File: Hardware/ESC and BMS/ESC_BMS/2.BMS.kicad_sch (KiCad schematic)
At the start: 46 parts, among them Q10 NTD25P03LT4G, Q8 NTD25P03LT4G, Q9 NMOS, SW2 SW_SPST, U12 BQ2969T, U13 74AUC2G08, U14 TPS25926, U16 BQ2057

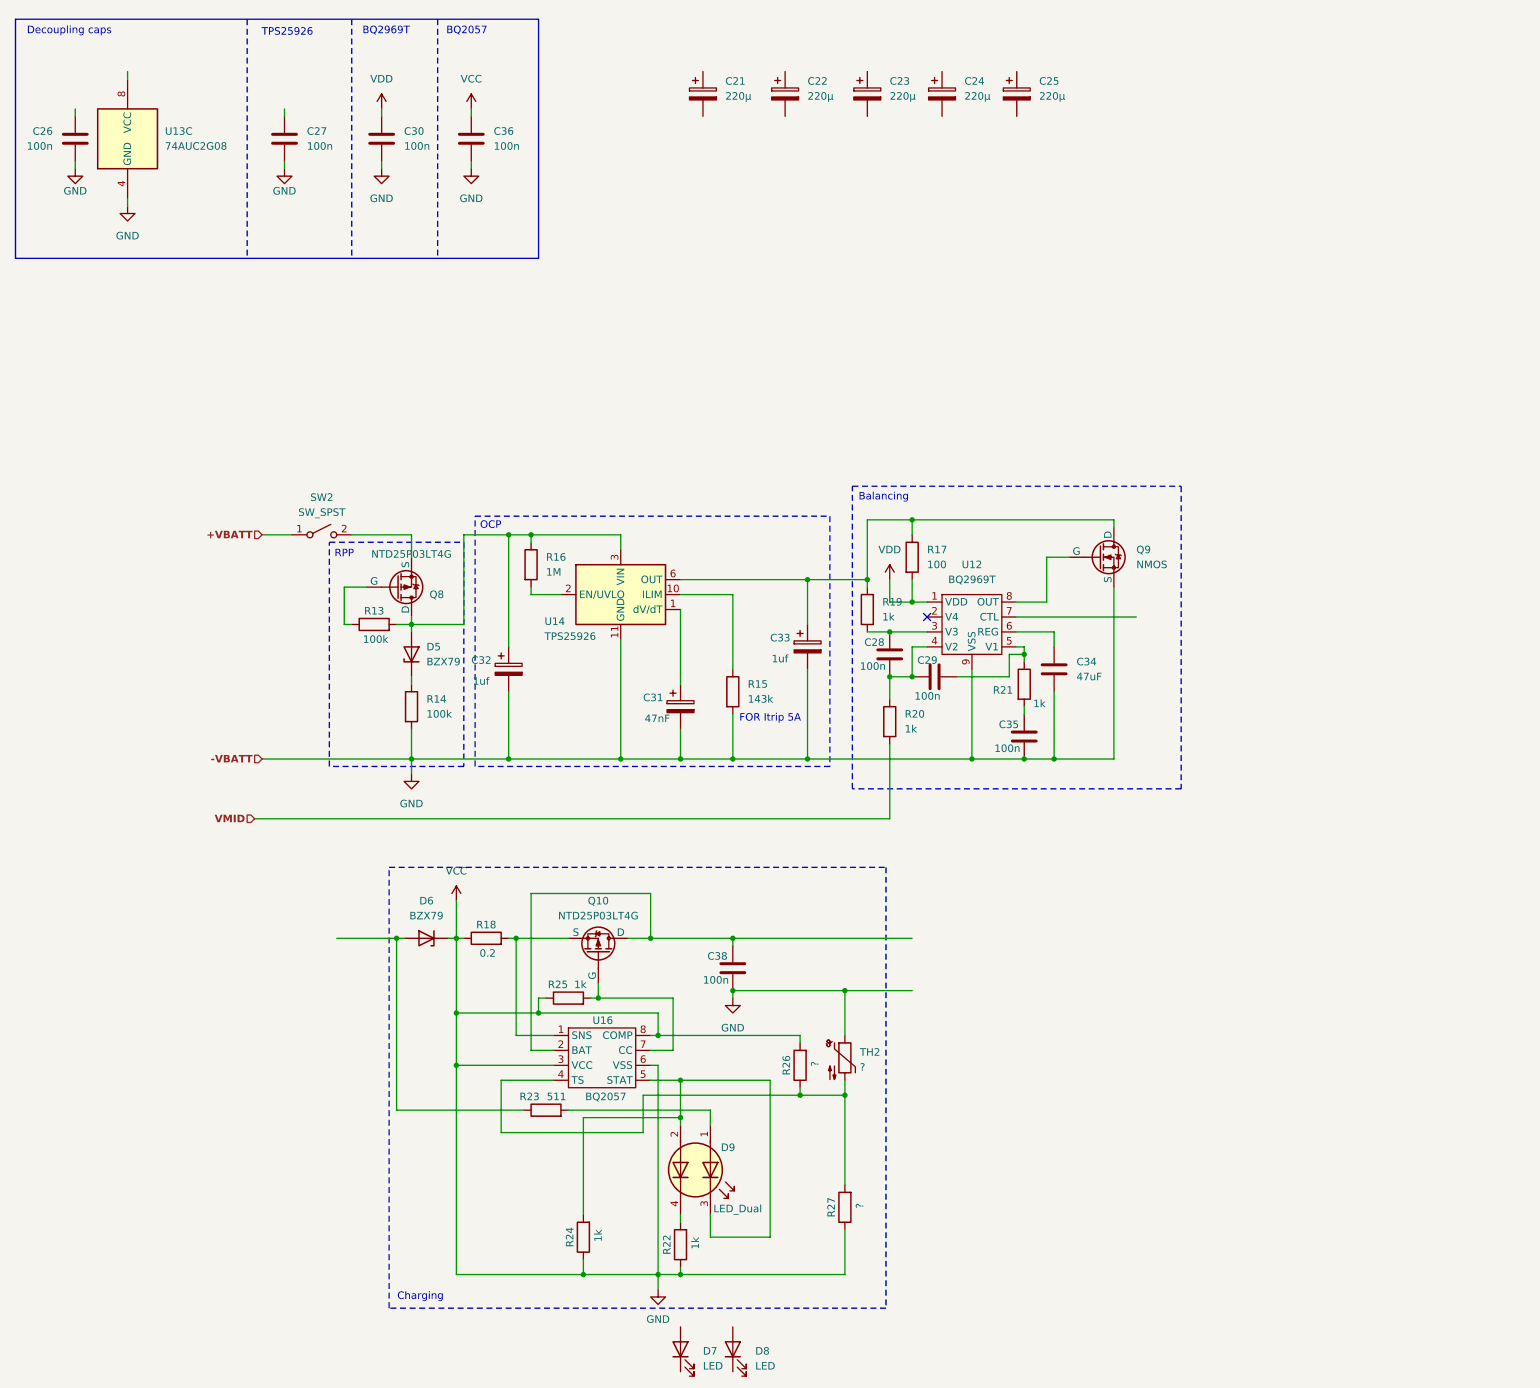
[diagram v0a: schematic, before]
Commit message: more BMS
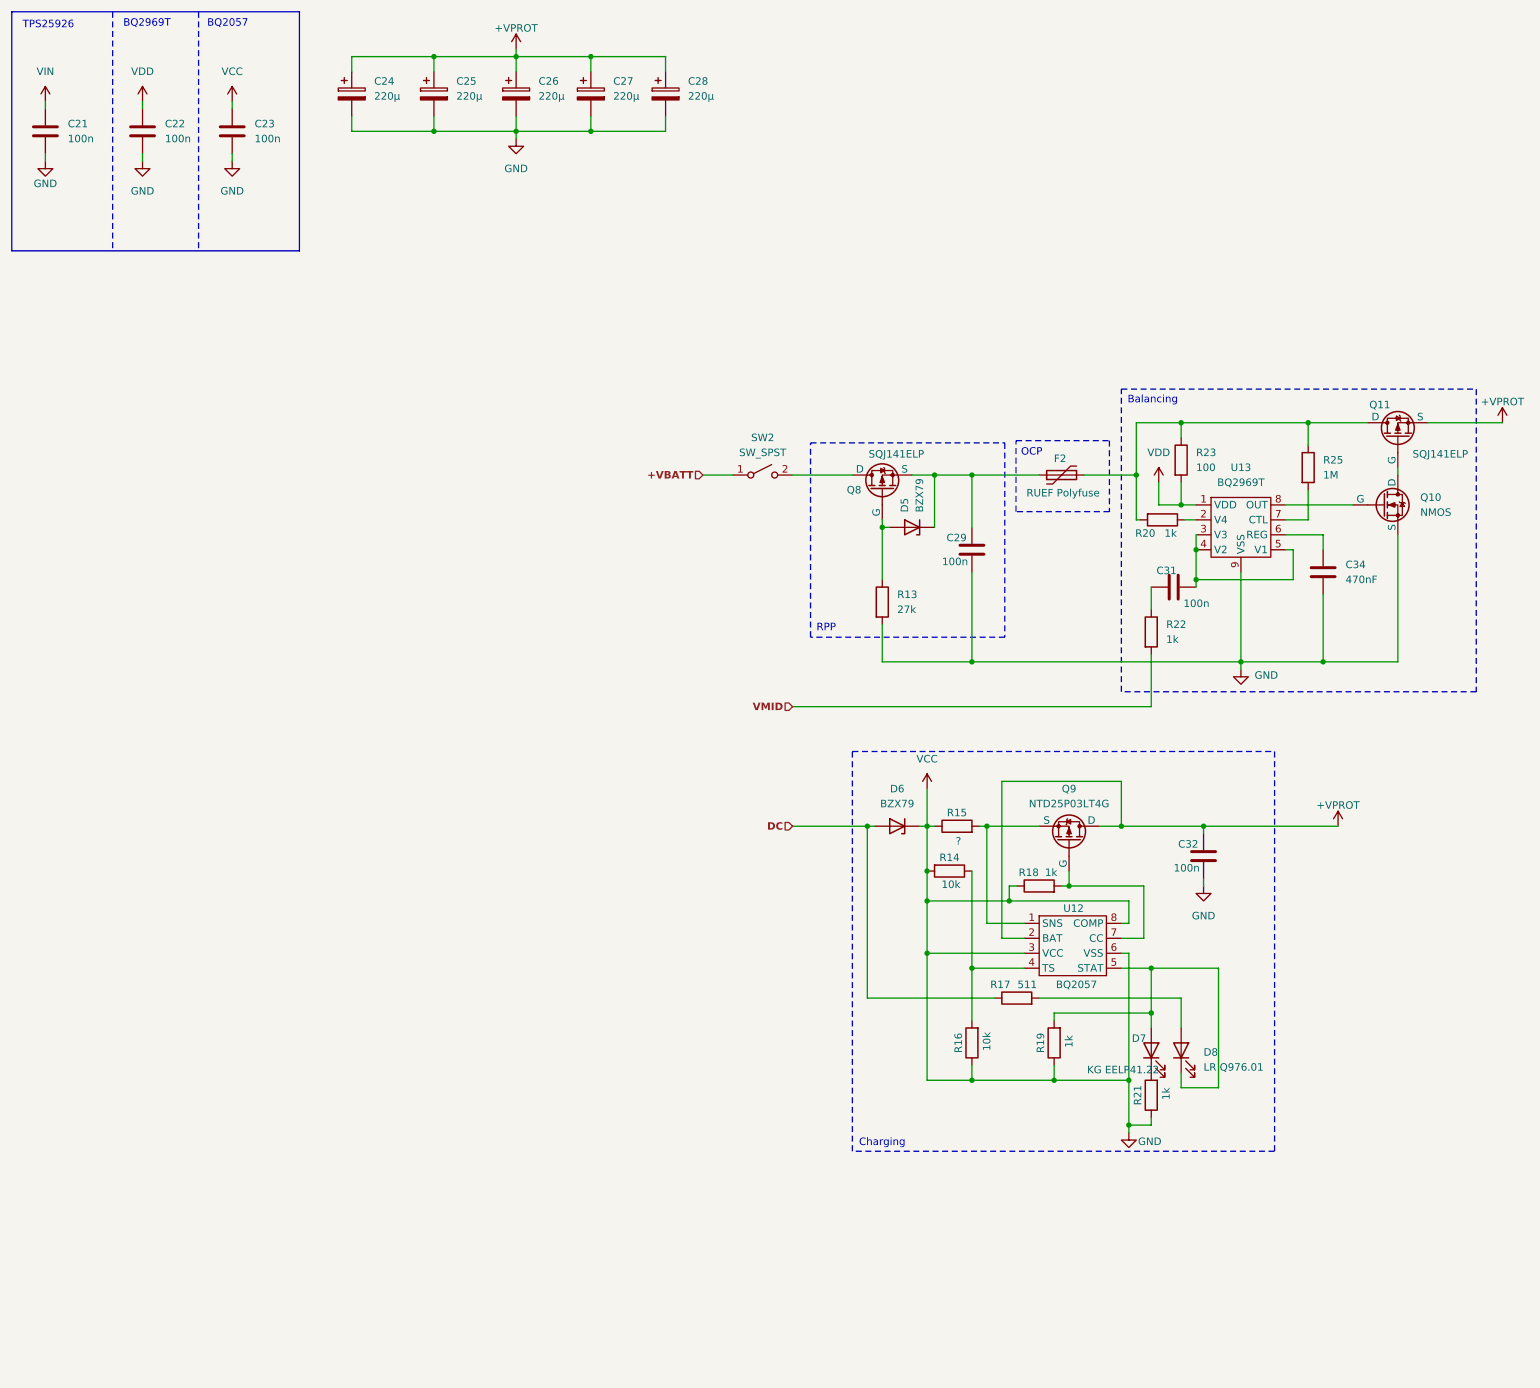
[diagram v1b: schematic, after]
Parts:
- removed C26, C28, C35: 100n, Capacitor_SMD:C_0603_1608Metric, symbol Device:C
- removed C31: 47nF, symbol Device:C_Polarized
- removed C32, C33: 1uf, symbol Device:C_Polarized
- removed D9: LED_Dual, symbol Device:LED_Dual_AAKK
- removed R13: 100k, symbol Device:R
- removed R15: 143k, symbol Device:R
- removed R21: 1k, symbol Device:R
- removed R26, R27: ?, symbol Device:R
- removed TH2: ?, symbol Device:Thermistor_NTC
- removed U13: 74AUC2G08, Package_SO:SSOP-8_2.95x2.8mm_P0.65mm, symbol 74xGxx:74AUC2G08
- removed U14: TPS25926, Package_SON:VSON-10-1EP_3x3mm_P0.5mm_EP1.65x2.4mm_ThermalVias, symbol Power_Management:TPS2592xx
- added C29: 100n, Capacitor_SMD:C_0603_1608Metric, symbol Device:C
- added F2: RUEF Polyfuse, Resistor_THT:R_Axial_DIN0207_L6.3mm_D2.5mm_P10.16mm_Horizontal, symbol Device:Polyfuse
- added Q11: SQJ141ELP, symbol Simulation_SPICE:PMOS
- added R14: 10k, symbol Device:R
- added R25: 1M, symbol Device:R
- C34: value 47uF -> 470nF
- D7: value LED -> KG EELP41.22
- D8: value LED -> LR Q976.01
- Q8: value NTD25P03LT4G -> SQJ141ELP
- R13: renamed from R14; value 100k -> 27k
- R15: renamed from R18; value 0.2 -> ?
- R16: value 1M -> 10k
- renumbered C27 to C21, C30 to C22, C36 to C23, C21 to C24, C22 to C25, C23 to C26, C24 to C27, C25 to C28, C29 to C31, C38 to C32, Q9 to Q10, Q10 to Q9, R23 to R17, R25 to R18, R24 to R19, R19 to R20, R22 to R21, R20 to R22, R17 to R23, U16 to U12, U12 to U13
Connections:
- net GND: now also C24.2, C25.2, C26.2, C27.2, C28.2, R16.1, C29.2, R14.2
- net +VPROT: now reaches C24.1
- net +VPROT: now also C25.1, C26.1, C27.1, C28.1, C32.1, Q9.1 (D), U12.2 (BAT), Q11.3 (S)
- net at U12.4 (TS): now also R16.2, R14.1
- net at R21.2: now also D7.1 (K)
- net at R20.2, R23.1: now also F2.2, Q11.1 (D), R25.1; no longer Q10.1 (D)
- net at Q8.3 (S): now also D5.1 (K), C29.1, F2.1; no longer SW2.2 (B)
- net at D8.1 (K): now also D7.2 (A), R19.2, U12.5 (STAT)
- net at D8.2 (A): now also R17.2
- net VIN: now reaches C21.1
- net at U13.3 (V3): now also C31.2, U13.4 (V2), U13.5 (V1); no longer R20.1
- net at C31.1, R22.1: no longer U13.4 (V2)
- net at R13.1: now also D5.2 (A), Q8.2 (G); no longer D5.1 (K)
- net DC: now reaches D6.2 (A), R17.1
- net at U13.2 (V4): now also R20.1
- net at U13.7 (CTL): now also R25.2
- new net: Q10.1 (D), Q11.2 (G)
- new net: Q8.1 (D), SW2.2 (B)
- no-connect marks 1 -> 0
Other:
- note removed: "Decoupling caps"
- note removed: "FOR Itrip 5A"
- moved on the sheet: C21, C22, C23, C24, C25, C26, C27, C28, C31, C32, C34, D5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
